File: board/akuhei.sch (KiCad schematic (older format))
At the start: 23 parts, among them J1 CLOCKPORT, J2 I2C, J3 AUXCLK, J4 JTAG, U1 XC9536XL-5VQG44C, U2 PCA9564, U3 TLV70233DBV

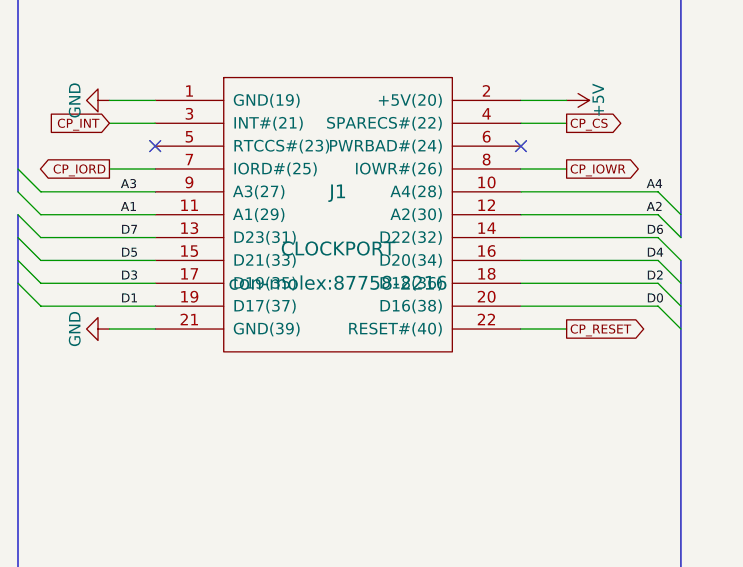
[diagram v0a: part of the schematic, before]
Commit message: Finishing touches...
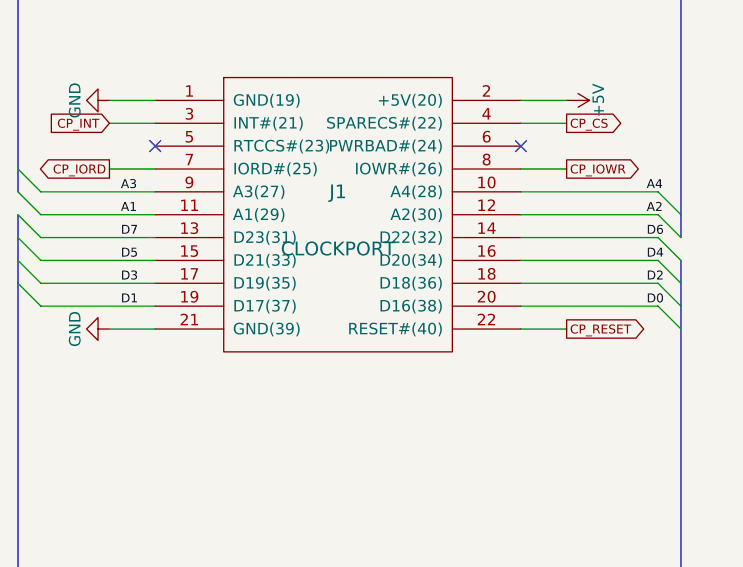
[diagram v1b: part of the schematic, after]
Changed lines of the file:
@@
 EESchema Schematic File Version 2
-LIBS:akuhei-rescue
 LIBS:power
 LIBS:device
@@
 F 0 "J1" H 2300 2400 60  0000 C CNN
 F 1 "CLOCKPORT" H 2300 2150 60  0000 C CNN
-F 2 "con-molex:87758-2216" H 2300 2000 60  0000 C CNN
+F 2 "con-molex:87758-2216" H 2300 2000 60  0001 C CNN
 F 3 "" H 2300 2000 60  0000 C CNN
 	1    2300 2300
